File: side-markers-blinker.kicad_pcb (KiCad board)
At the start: 2 copper layers, 69 x 66.5 mm, 32 parts, among them J5 Conn_01x07_Socket, Q1 IRF540N, Q2 BC546, Q3 BC546, Q4 IRF540N, Q5 BC546, Q6 BC546

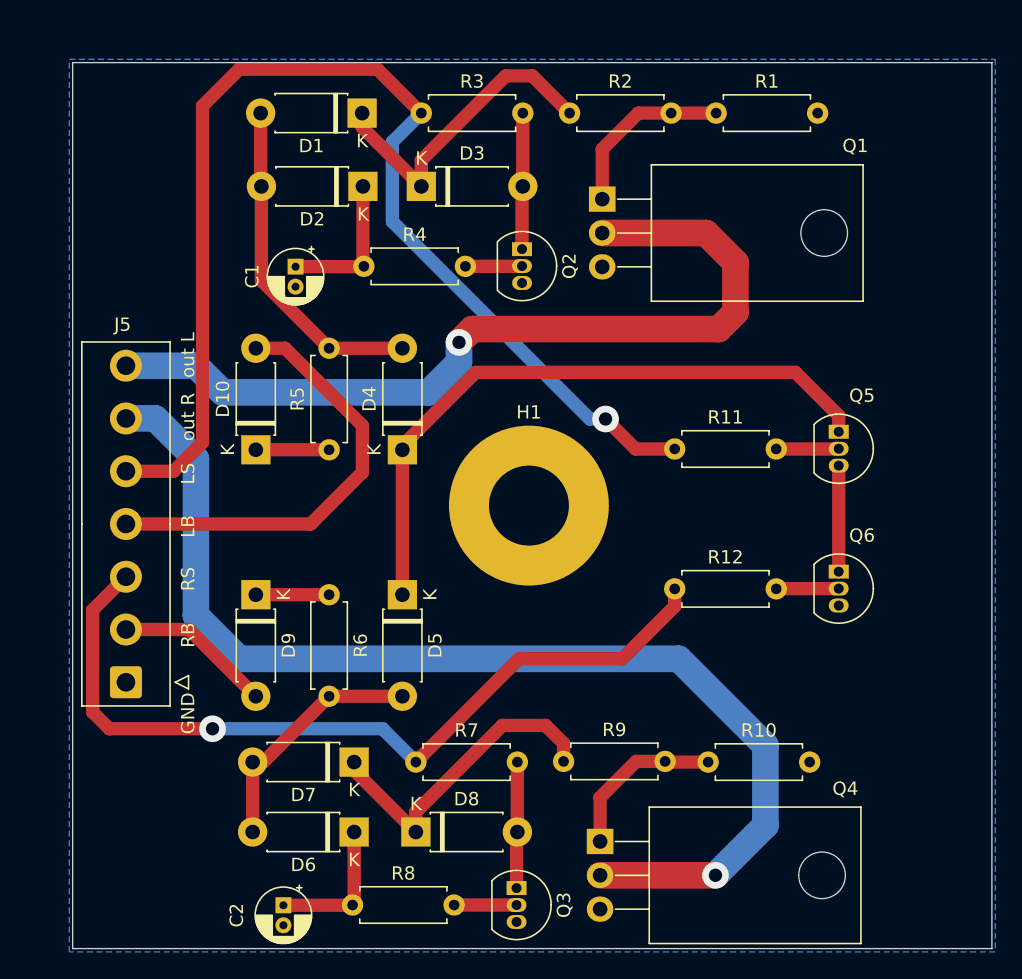
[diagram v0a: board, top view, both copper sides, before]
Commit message: Redesigned pcb to use p channel mosfets.
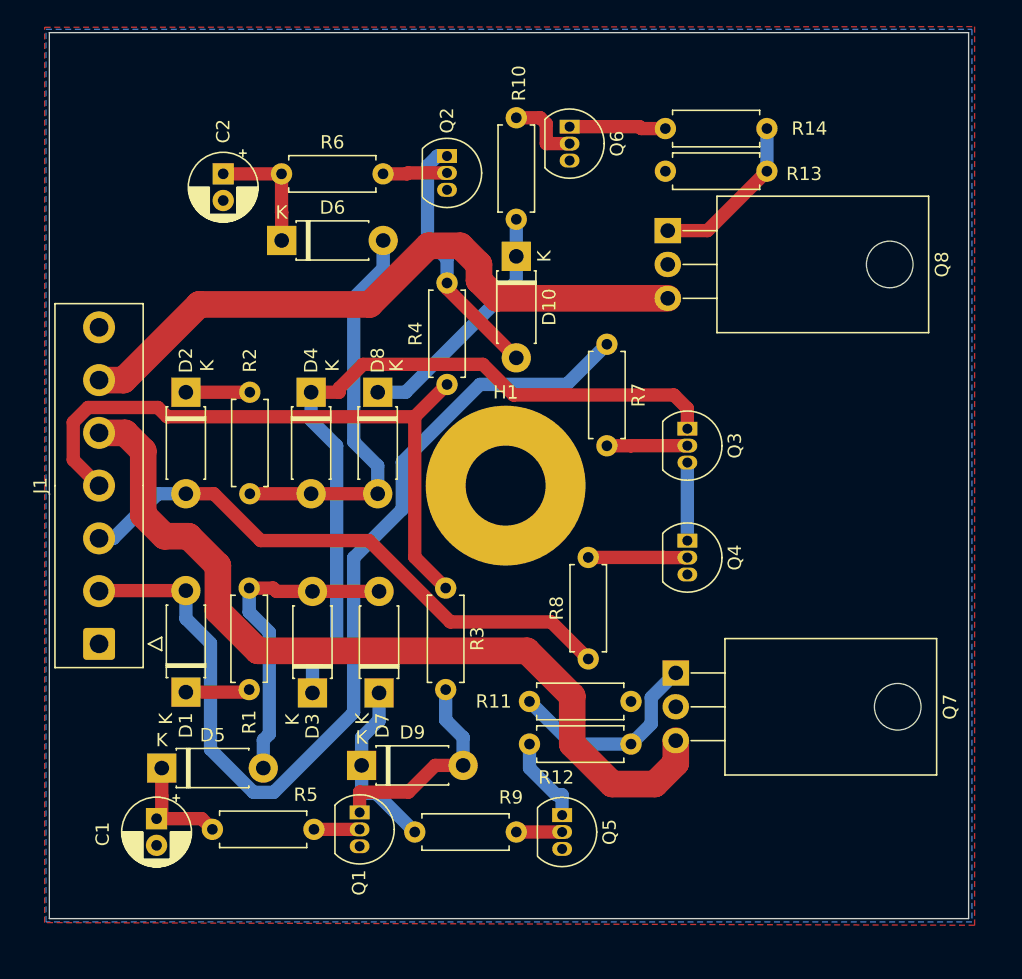
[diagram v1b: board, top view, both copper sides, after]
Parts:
- removed J5: Conn_01x07_Socket, Connector_TE-Connectivity:TE_826576-7_1x07_P3.96mm_Vertical
- added J1: Conn_01x07_Socket, Connector_TE-Connectivity:TE_826576-7_1x07_P3.96mm_Vertical, F.Cu at (113.5, 108.1)
- added Q7: IRF4905, Package_TO_SOT_THT:TO-220-3_Horizontal_TabDown, F.Cu at (156.8, 110.3)
- added Q8: IRF4905, Package_TO_SOT_THT:TO-220-3_Horizontal_TabDown, F.Cu at (156.2, 77.1)
- added R13: 10k, Resistor_THT:R_Axial_DIN0207_L6.3mm_D2.5mm_P7.62mm_Horizontal, F.Cu at (163.6, 72.7)
- added R14: 10k, Resistor_THT:R_Axial_DIN0207_L6.3mm_D2.5mm_P7.62mm_Horizontal, F.Cu at (163.6, 69.5)
- C1, C2: footprint Capacitor_THT:CP_Radial_D4.0mm_P1.50mm -> Capacitor_THT:CP_Radial_D5.0mm_P2.00mm
- Q1, Q4: value IRF540N -> BC547; footprint Package_TO_SOT_THT:TO-220-3_Horizontal_TabDown -> Package_TO_SOT_THT:TO-92_Inline
- Q2, Q3, Q5, Q6: value BC546 -> BC547
- R1, R10: value 100k -> 10k
- R11, R12, R5, R6: value 1k -> 10k
- R2, R9: value 50k -> 10k
- moved R1 55.7 mm to (124.8, 111.6), turned to 90 degrees
- moved C2 55.1 mm to (122.8, 72.8)
- moved Q1 49.5 mm to (133.0, 120.8)
- moved D1 45.4 mm to (120.0, 111.8), turned to 90 degrees
- moved D6 44.7 mm to (127.2, 77.8), turned to 0 degrees
- moved R10 43.2 mm to (144.8, 76.3), turned to 90 degrees
- moved C1 42.7 mm to (117.8, 121.2)
- moved Q6 39.0 mm to (148.8, 69.3)
- moved D3 38.9 mm to (129.5, 111.8), turned to 90 degrees
- moved Q3 36.8 mm to (157.6, 92.0)
- moved R3 35.7 mm to (139.5, 103.9), turned to -90 degrees
- moved Q5 35.5 mm to (148.2, 121.0)
- moved R7 34.5 mm to (151.6, 85.6), turned to -90 degrees
- moved D8 33.1 mm to (134.4, 89.2), turned to -90 degrees
- moved R2 31.9 mm to (124.8, 89.2), turned to -90 degrees
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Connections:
- C1 pad 1: Net-(D2-K) -> Net-(D5-K)
- D1 pad 2: Net-(D1-A) -> Blinker signal R input
- D10 pad 2: Blinker signal L -> Net-(D10-A)
- D2 pad 2: Net-(D1-A) -> Blinker signal L input
- D3 pad 1: Net-(D1-K) -> AND gate
- D4 pad 2: Net-(D1-A) -> Net-(D4-A)
- D5 pad 1: AND gate -> Net-(D5-K)
- D5 pad 2: Net-(D5-A) -> Net-(D3-A)
- D6 pad 2: Net-(D5-A) -> Net-(D4-A)
- D7 pad 2: Net-(D5-A) -> Net-(D3-A)
- D8 pad 1: Net-(D7-K) -> Net-(D10-K)
- D8 pad 2: Net-(D8-A) -> Net-(D4-A)
- D9 pad 1: Net-(D9-K) -> Net-(D7-K)
- D9 pad 2: Blinker signal R -> Net-(D9-A)
- Q1 pad 1: Net-(Q1-G) -> Net-(D9-A)
- Q1 pad 2: Side marker lamp GND L -> Net-(Q1-B)
- Q2 pad 1: Net-(D3-A) -> Net-(D10-A)
- Q3 pad 1: Net-(D8-A) -> AND gate
- Q3 pad 3: GND -> Net-(Q3-E)
- Q4 pad 1: Net-(Q4-G) -> Net-(Q3-E)
- Q4 pad 2: Side marker lamp GND R -> Net-(Q4-B)
- Q5 pad 1: AND gate -> Net-(Q5-C)
- Q5 pad 3: Net-(Q5-E) -> GND
- Q6 pad 1: Net-(Q5-E) -> Net-(Q6-C)
- R1 pad 1: Net-(Q1-G) -> Net-(D1-K)
- R1 pad 2: GND -> Net-(D3-A)
- R10 pad 1: Net-(Q4-G) -> Net-(D10-K)
- R10 pad 2: GND -> Net-(Q6-B)
- R11 pad 1: Side marker signal L -> Net-(Q7-G)
- R11 pad 2: Net-(Q5-B) -> +24v when igniton on
- R12 pad 1: Side marker signal R -> Net-(Q7-G)
- R12 pad 2: Net-(Q6-B) -> Net-(Q5-C)
- R2 pad 1: Net-(D1-K) -> Net-(D2-K)
- R2 pad 2: Net-(Q1-G) -> Net-(D4-A)
- R3 pad 1: Side marker signal L -> Side markers signal input
- R3 pad 2: Net-(D3-A) -> Net-(D9-A)
- R4 pad 1: Net-(D2-K) -> Side markers signal input
- R4 pad 2: Net-(Q2-B) -> Net-(D10-A)
- R5 pad 1: Net-(D10-K) -> Net-(D5-K)
- R5 pad 2: Net-(D1-A) -> Net-(Q1-B)
- R6 pad 1: Net-(D9-K) -> Net-(D6-K)
- R6 pad 2: Net-(D5-A) -> Net-(Q2-B)
- R7 pad 1: Side marker signal R -> Blinker signal R input
- R7 pad 2: Net-(D8-A) -> Net-(Q3-B)
- R8 pad 1: Net-(D6-K) -> Blinker signal L input
- R8 pad 2: Net-(Q3-B) -> Net-(Q4-B)
- R9 pad 2: Net-(Q4-G) -> Net-(Q5-B)
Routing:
- net Side marker signal L: track 88.1 -> 0.00 mm, vias 1 -> 0
- net Side marker lamp GND R: track 85.0 -> 0.00 mm, vias 1 -> 0
- net Blinker signal R input: track 0.00 -> 73.1 mm
- net Side marker lamp GND L: track 64.6 -> 0.00 mm, vias 1 -> 0
- net Side marker lamp +24 R output: track 0.00 -> 63.5 mm
- net Side marker signal R: track 62.6 -> 0.00 mm, vias 1 -> 0
- net Side marker lamp +24 L output: track 0.00 -> 49.2 mm
- net Side markers signal input: track 0.00 -> 49.2 mm
- net Blinker signal L input: track 0.00 -> 43.2 mm
- net Blinker signal L: track 33.3 -> 0.00 mm
- net Net-(D4-A): track 0.00 -> 30.3 mm
- net Net-(D1-A): track 25.3 -> 0.00 mm
- net Net-(D1-K): track 24.2 -> 4.83 mm
- net Net-(D10-A): track 0.00 -> 18.9 mm
- net Net-(D5-A): track 18.5 -> 0.00 mm
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- added copper zone on F.Cu, net +24v when igniton on
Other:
- board text removed: "GND"
- board text removed: "LB"
- board text removed: "LS"
- board text removed: "RB"
- board text removed: "RS"
- board text removed: "out L"
- board text removed: "out R"
